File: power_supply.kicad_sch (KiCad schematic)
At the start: 18 parts, among them J1 Разъём к автомобилю 2x16 (32 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, U6 MC78M05CDTG, U7 AMS1117-3.3

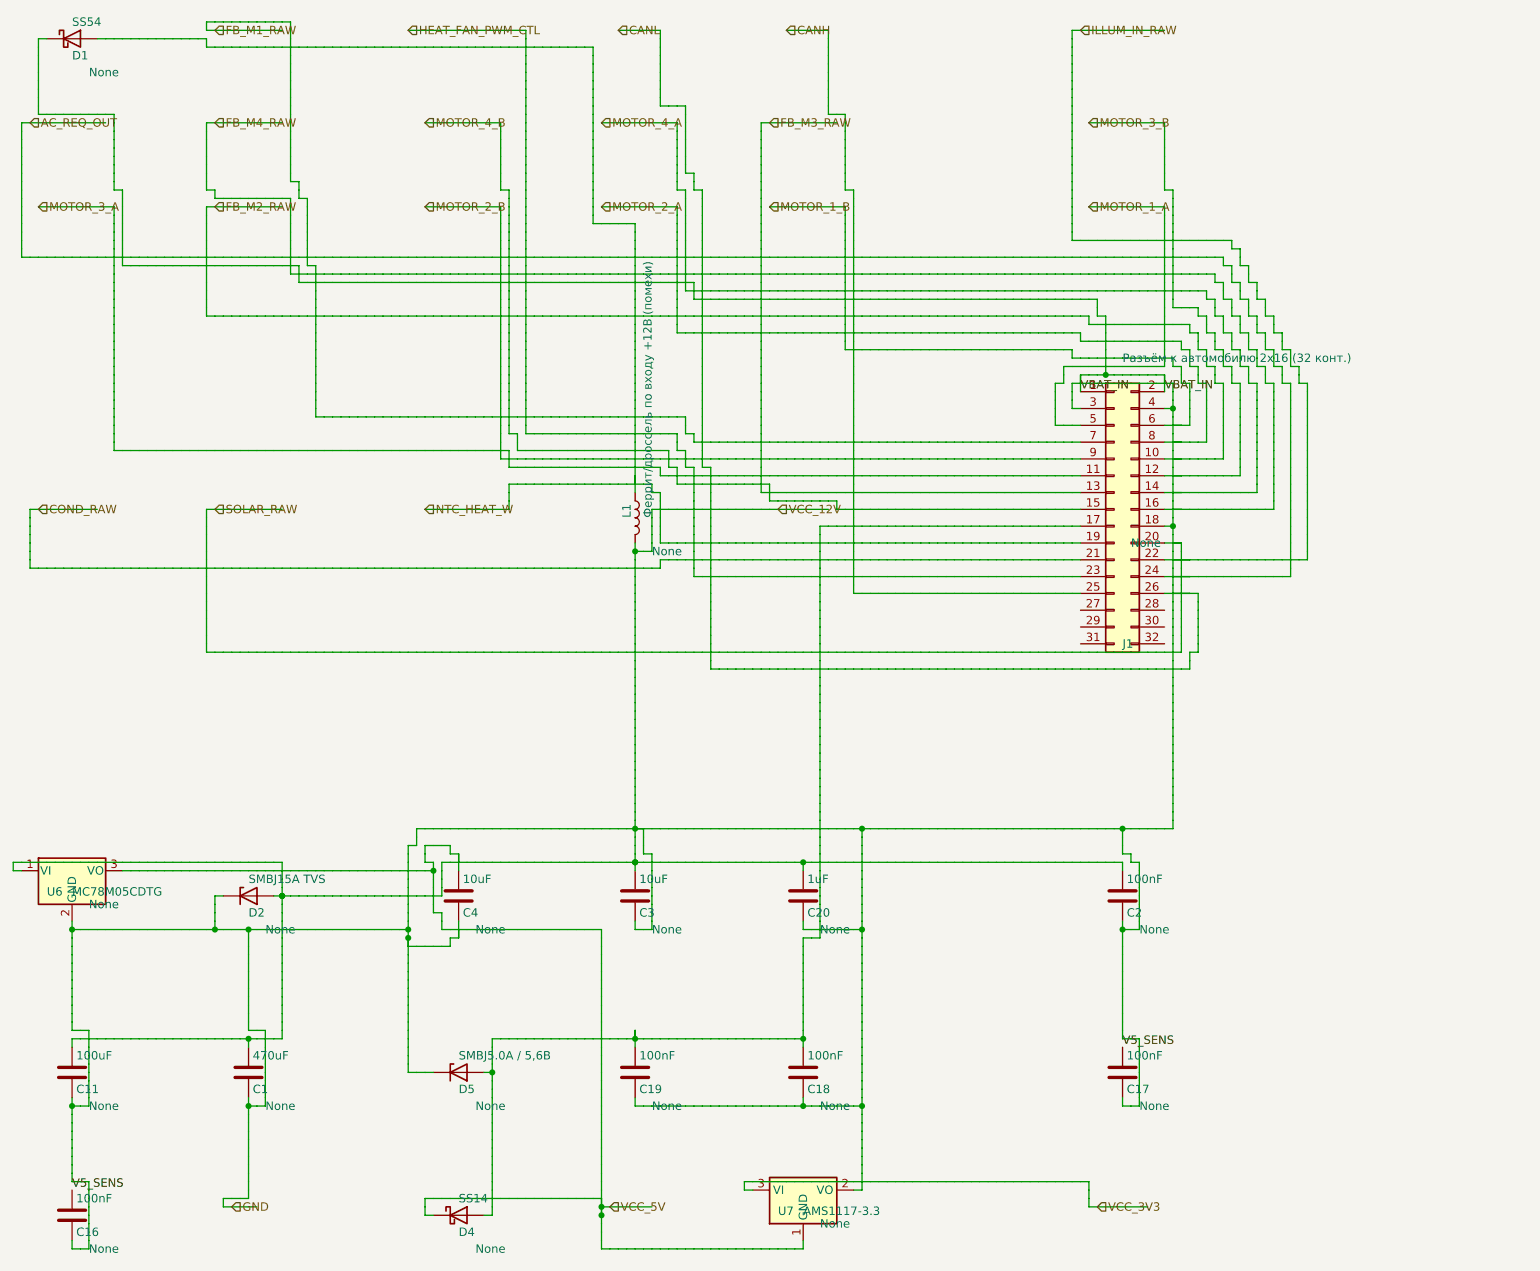
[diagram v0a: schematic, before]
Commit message: рефакторинг проекта и начала прогона тестов
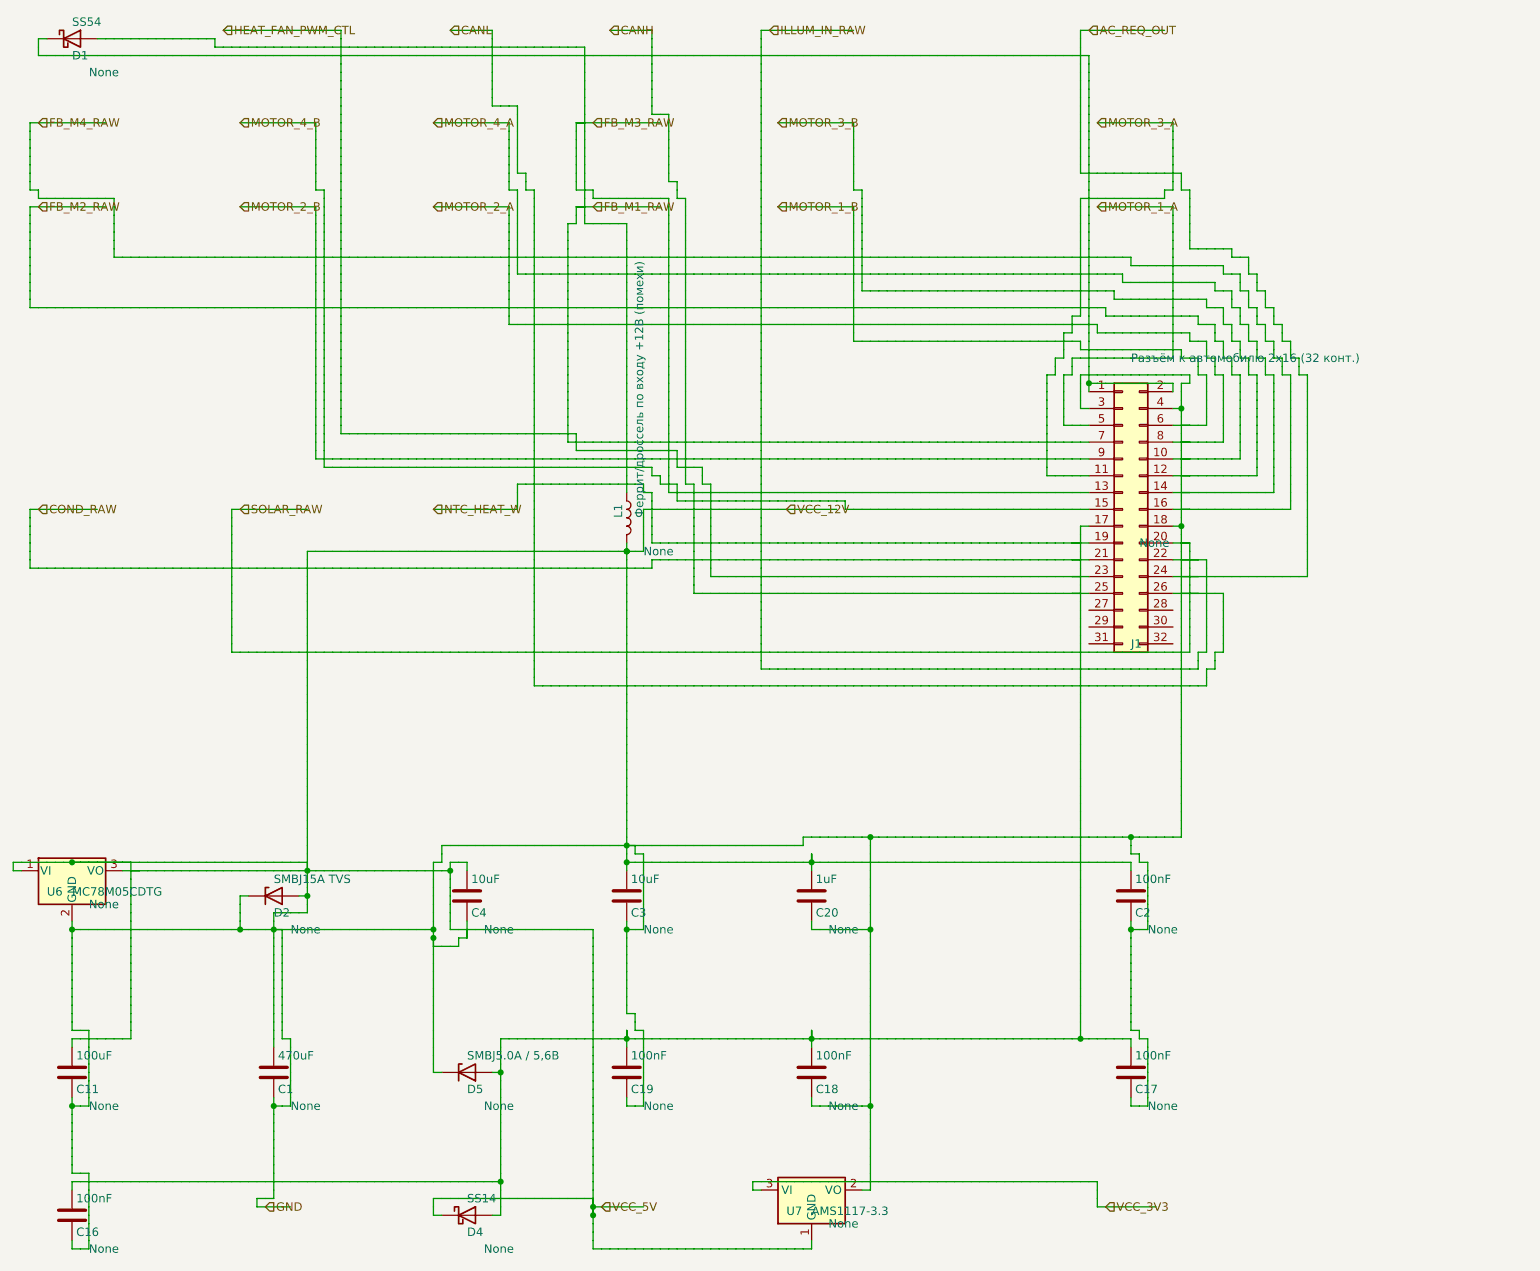
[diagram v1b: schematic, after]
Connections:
- net V5_SENS is gone; now on net AC_REQ_OUT: C16.1, C17.1
